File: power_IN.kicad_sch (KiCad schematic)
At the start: 26 parts, among them J1 Conn_01x02, J2 +VDC, J3 -VDC, J4 58-8 OUTPUT, U1 LM2931-5.0_TO220, U2 XC6206PxxxMR, U3 XC6206PxxxMR, U4 LM2931-5.0_TO220, U5 XC6206PxxxMR, U6 XC6206PxxxMR, U7 LM2931-5.0_TO220

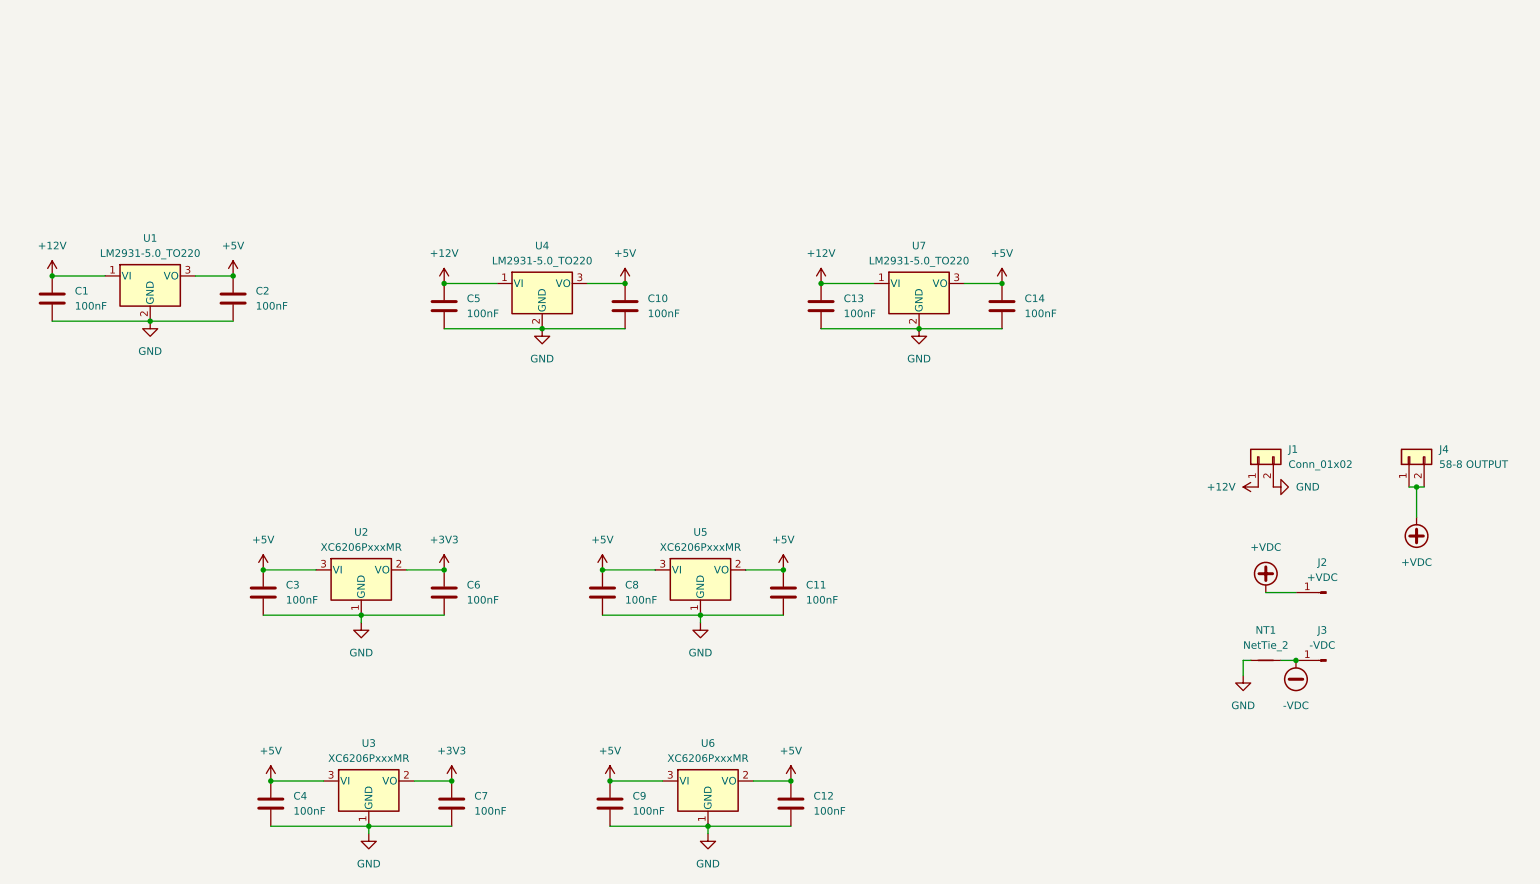
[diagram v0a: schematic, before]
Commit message: pcb geçiş
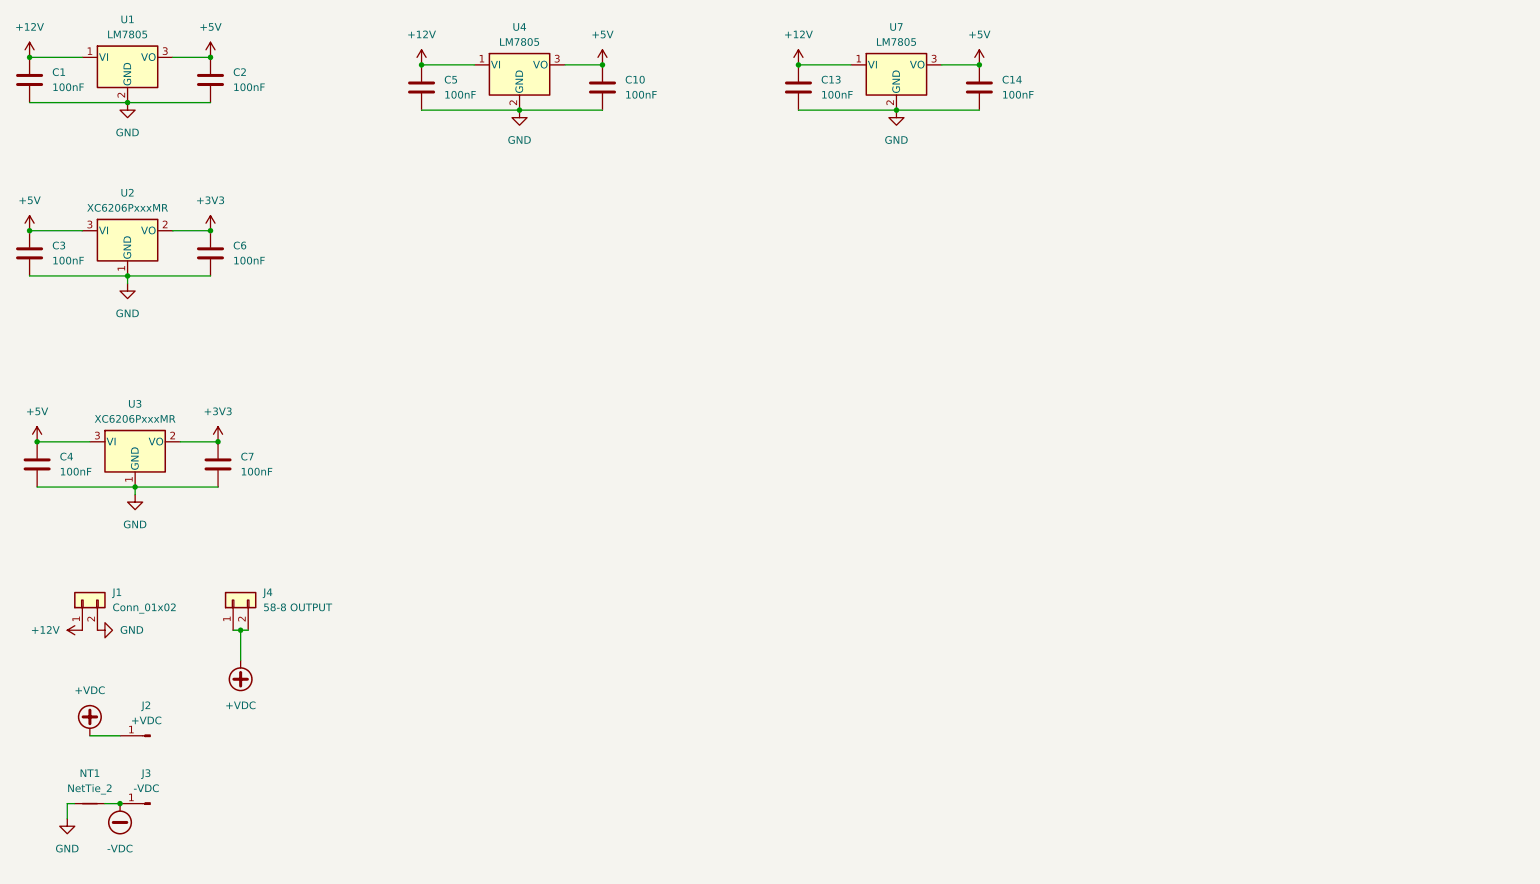
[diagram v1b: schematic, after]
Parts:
- removed C11, C12, C8, C9: 100nF, Capacitor_SMD:C_1210_3225Metric_Pad1.33x2.70mm_HandSolder, symbol Device:C
- removed U5, U6: XC6206PxxxMR, Package_TO_SOT_SMD:SOT-23-3, symbol Regulator_Linear:XC6206PxxxMR
- J1: footprint (none) -> TerminalBlock_RND:TerminalBlock_RND_205-00001_1x02_P5.00mm_Horizontal
- J4: footprint (none) -> TerminalBlock_Ningbo-Kagnex:TerminalBlock_Ningbo-Kagnex_HB9500_1x02_P9.5mm
- NT1: footprint (none) -> NetTie:NetTie-2_SMD_Pad2.0mm
- U1, U4, U7: value LM2931-5.0_TO220 -> LM7805
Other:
- moved on the sheet: C1, C10, C13, C14, C2, C3, C4, C5, C6, C7, J1, J2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
